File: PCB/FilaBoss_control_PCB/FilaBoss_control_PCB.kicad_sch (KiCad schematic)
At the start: 35 parts, among them J1 Conn_01x04_Encoder, J10 Screw_Terminal_01x02, J11 SCL/SDA, J12 Screw_Terminal_01x02, J13 Screw_Terminal_01x02, J14 Conn_01x04_Encoder, J2 SPOOL, J3 PULLER, J4 RX/TX, J5 Barrel_Jack_SMD, J6 PinHeader_01x06_P2.54mm_Verti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, J7 Conn_01x04, J8 JST_2mm_3, J9 Conn_01x04_Pot, M1 Motor_DC, M2 Motor_DC, Q1 IRLZ44N, Q2 IRLZ44N, SW1 RotaryEncoder_Switch, U2 R-78E5.0-0.5, U3 R-78B12-2.0

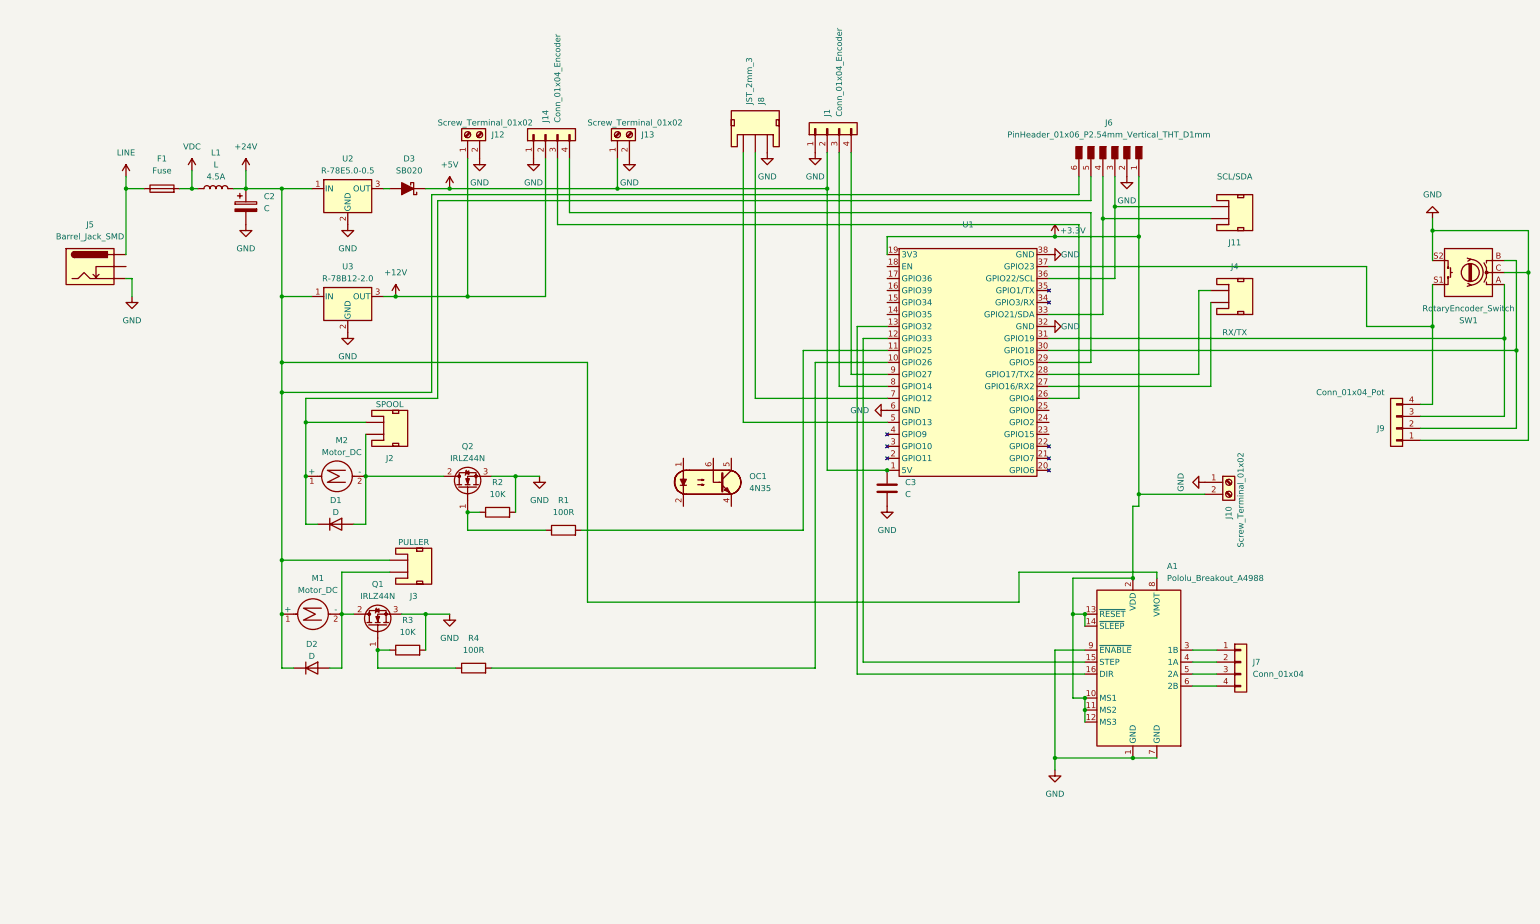
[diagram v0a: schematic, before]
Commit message: pcb
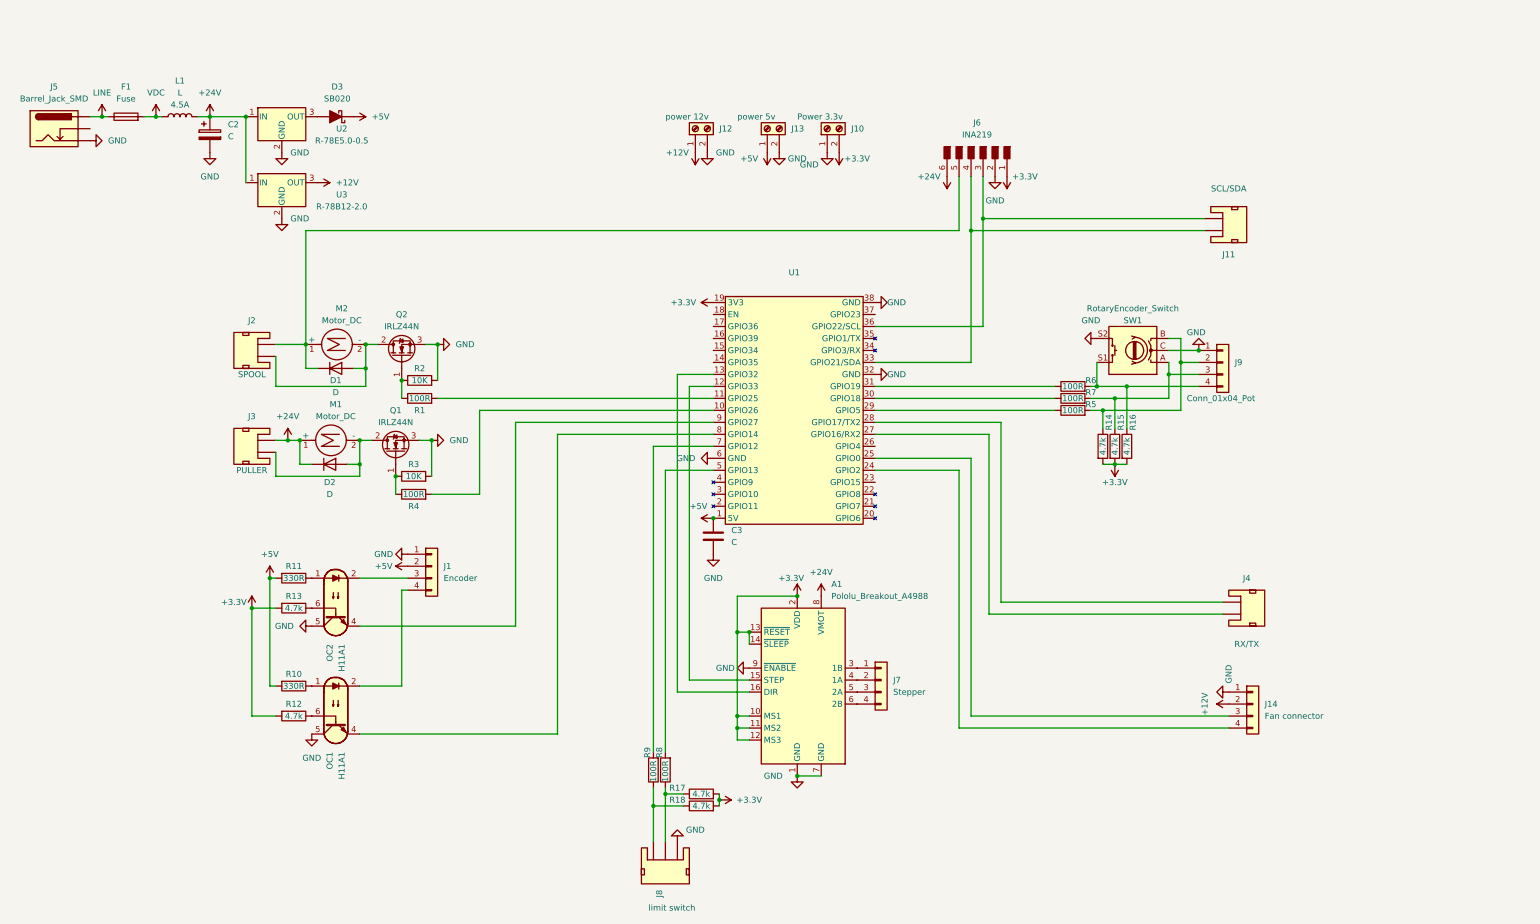
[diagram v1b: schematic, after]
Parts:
- removed OC1: 4N35, PCM_Package_DIP_AKL:DIP-6_W7.62mm_LongPads, symbol PCM_Optocoupler_AKL:4N35
- added OC1, OC2: H11A1, PCM_Package_DIP_AKL:DIP-6_W7.62mm_LongPads, symbol PCM_Optocoupler_AKL:H11A1
- added R10, R11: 330R, Resistor_THT:R_Axial_DIN0207_L6.3mm_D2.5mm_P10.16mm_Horizontal, symbol Device:R
- added R12, R13, R14, R15, R16, R17, R18: 4.7k, Resistor_THT:R_Axial_DIN0207_L6.3mm_D2.5mm_P10.16mm_Horizontal, symbol Device:R
- added R5, R6, R7, R8, R9: 100R, Resistor_THT:R_Axial_DIN0207_L6.3mm_D2.5mm_P10.16mm_Horizontal, symbol Device:R
- J1: value Conn_01x04_Encoder -> Encoder
- J10: value Screw_Terminal_01x02 -> Power 3.3v
- J12: value Screw_Terminal_01x02 -> power 12v
- J13: value Screw_Terminal_01x02 -> power 5v
- J14: value Conn_01x04_Encoder -> Fan connector
- J6: value PinHeader_01x06_P2.54mm_Vertical_THT_D1mm -> INA219
- J7: value Conn_01x04 -> Stepper
- J8: value JST_2mm_3 -> limit switch
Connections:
- net +24V: now also J3.2 (+); no longer J3.1 (-)
- net +3.3V: now also R12.2, R13.2, R14.2, R15.2, R16.2, R17.2, R18.2
- net +5V: now also R10.2, R11.2
- net GND: now also J8.3, OC1.5, OC2.5; no longer J8.1
- net at D1.1 (K), J6.5 (Pin_5), M2.1 (+): now also J2.2 (+); no longer J2.1 (-)
- net at D1.2 (A), M2.2 (-), Q2.2 (D): now also J2.1 (-); no longer J2.2 (+)
- net at D2.2 (A), M1.2 (-), Q1.2 (D): now also J3.1 (-); no longer J3.2 (+)
- net at J9.2 (Pin_2), SW1.B: now also R14.1, R5.2; no longer U1.30 (GPIO18)
- net at J9.3 (Pin_3), SW1.A: now also R15.1, R7.2; no longer U1.31 (GPIO19)
- net at J9.4 (Pin_4), SW1.S1: now also R16.1, R6.2; no longer U1.37 (GPIO23)
- net at U1.24 (GPIO2): now also J14.4 (Pin_4)
- net at U1.25 (GPIO0): now also J14.3 (Pin_3)
- net at U1.26 (GPIO4): no longer J14.3 (Pin_3)
- net at U1.29 (GPIO5): now also R5.1; no longer J14.4 (Pin_4)
- net at U1.5 (GPIO13): now also R8.2; no longer J8.3
- net at U1.7 (GPIO12): now also R9.2; no longer J8.2
- net at U1.8 (GPIO14): now also OC1.4; no longer J1.3 (Pin_3)
- net at J1.4 (Pin_4): now also OC1.2; no longer U1.9 (GPIO27)
- new net: R7.1, U1.30 (GPIO18)
- new net: OC1.1, R10.1
- new net: OC1.6, R12.1
- new net: J8.1, R18.1, R9.1
- new net: J8.2, R17.1, R8.1
- new net: R6.1, U1.31 (GPIO19)
- new net: OC2.4, U1.9 (GPIO27)
- new net: J1.3 (Pin_3), OC2.2
- new net: OC2.6, R13.1
- new net: OC2.1, R11.1
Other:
- moved on the sheet: A1, C2, C3, D1, D2, D3, F1, J1, J10, J11, J12, J13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
